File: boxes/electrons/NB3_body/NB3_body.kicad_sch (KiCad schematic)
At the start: 32 parts, among them J1 Conn_02x05_Counter_Clockwise, J10 Conn_02x03_Top_Bottom, J11 Conn_02x03_Top_Bottom, J12 Conn_02x03_Top_Bottom, J13 JST ZH 6-way Socket, J14 JST ZH 6-way Socket, J2 Conn_02x05_Counter_Clockwise, J3 Conn_02x05_Counter_Clockwise, J4 Conn_02x05_Counter_Clockwise, J5 Conn_02x05_Counter_Clockwise, J6 Conn_02x05_Counter_Clockwise, J7 Conn_02x05_Counter_Clockwise, J8 Conn_02x05_Counter_Clockwise, J9 JST SH 4-way Socket

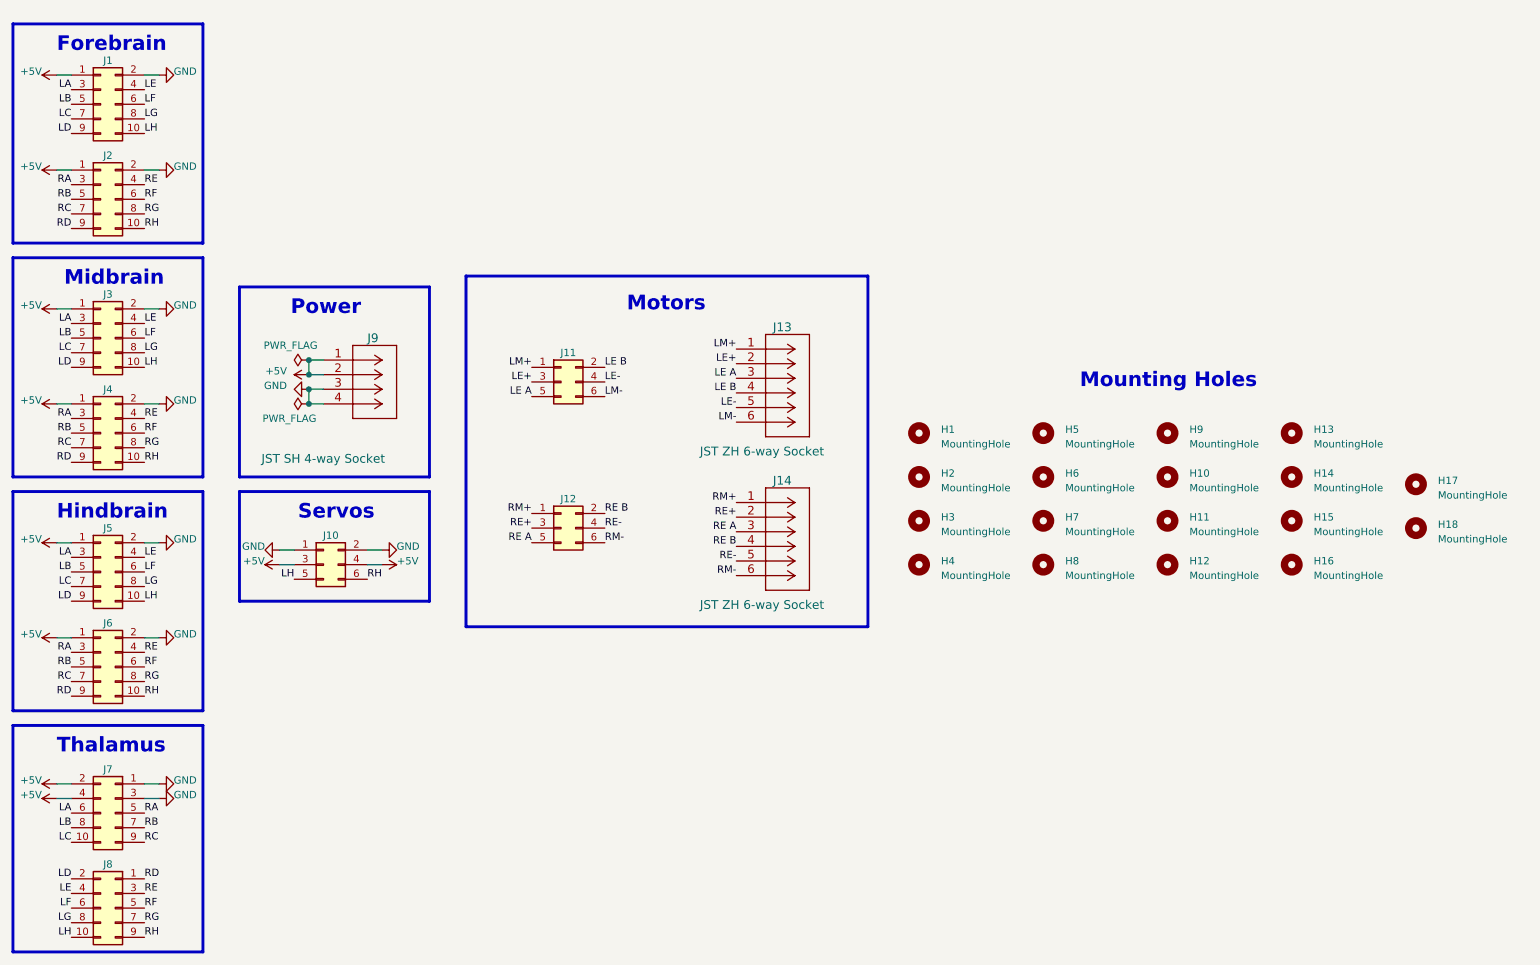
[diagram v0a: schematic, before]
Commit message: Work on NB£_body PCB
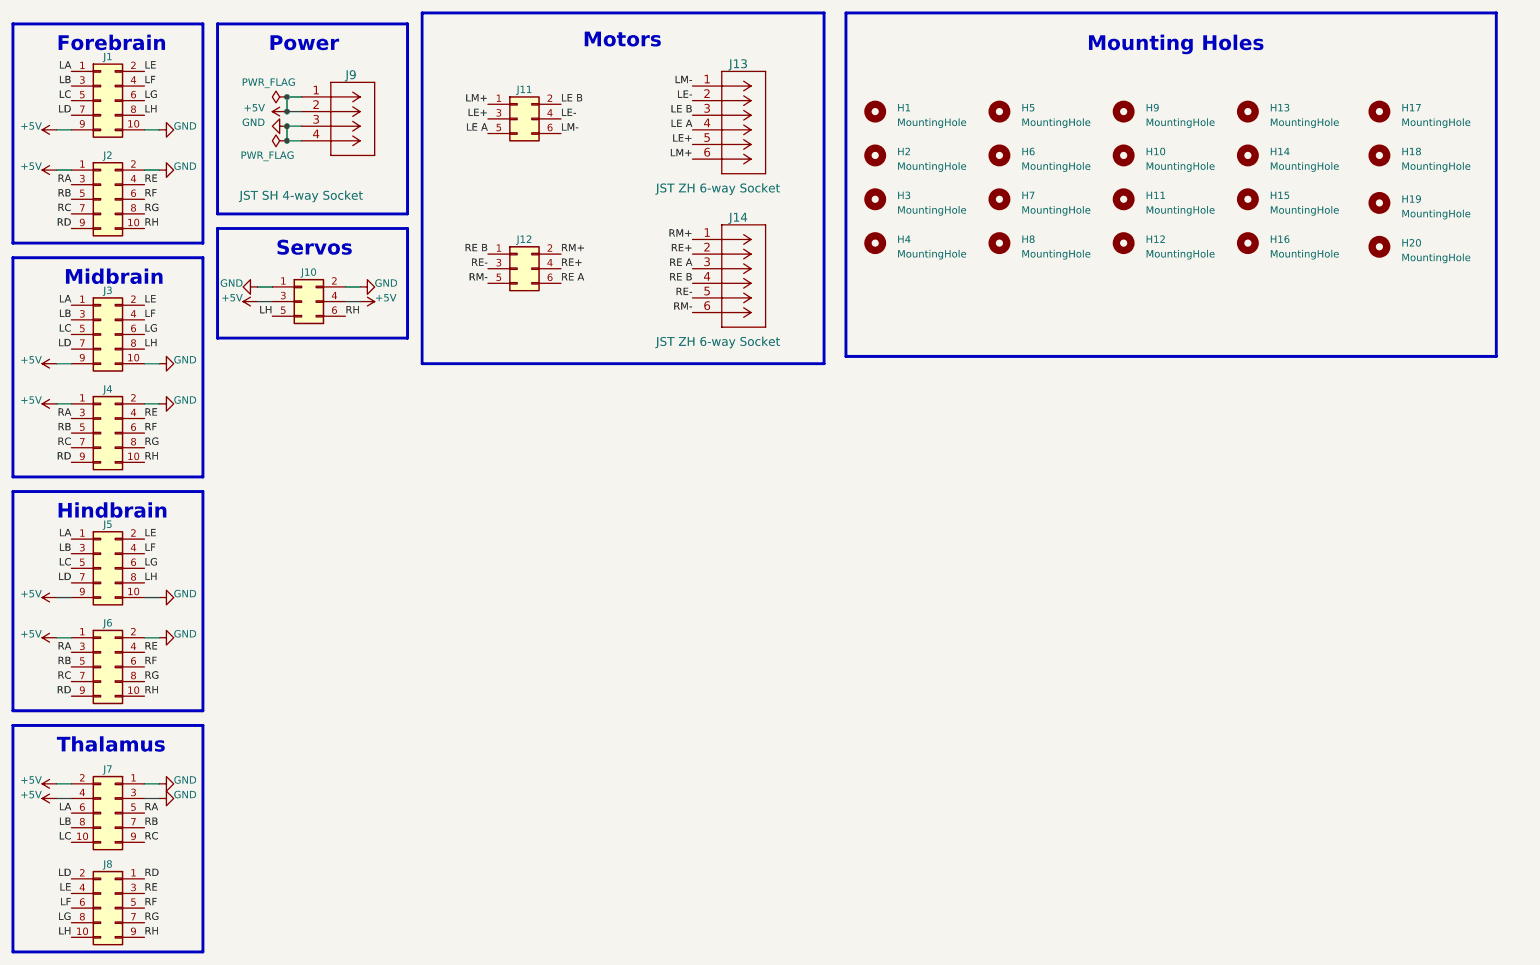
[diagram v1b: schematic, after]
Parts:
- added H19, H20: MountingHole, MountingHole:MountingHole_2.7mm_M2.5_ISO7380_Pad, symbol Mechanical:MountingHole
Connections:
- net +5V: now also J1.9 (Pin_9), J3.9 (Pin_9), J5.9 (Pin_9); no longer J1.1 (Pin_1), J3.1 (Pin_1), J5.1 (Pin_1)
- net GND: now also J1.10 (Pin_10), J3.10 (Pin_10), J5.10 (Pin_10); no longer J1.2 (Pin_2), J3.2 (Pin_2), J5.2 (Pin_2)
- net LA: now also J1.1 (Pin_1), J3.1 (Pin_1), J5.1 (Pin_1); no longer J1.3 (Pin_3), J3.3 (Pin_3), J5.3 (Pin_3)
- net LB: now also J1.3 (Pin_3), J3.3 (Pin_3), J5.3 (Pin_3); no longer J1.5 (Pin_5), J3.5 (Pin_5), J5.5 (Pin_5)
- net LC: now also J1.5 (Pin_5), J3.5 (Pin_5), J5.5 (Pin_5); no longer J1.7 (Pin_7), J3.7 (Pin_7), J5.7 (Pin_7)
- net LD: now also J1.7 (Pin_7), J3.7 (Pin_7), J5.7 (Pin_7); no longer J1.9 (Pin_9), J3.9 (Pin_9), J5.9 (Pin_9)
- net LE: now also J1.2 (Pin_2), J3.2 (Pin_2), J5.2 (Pin_2); no longer J1.4 (Pin_4), J3.4 (Pin_4), J5.4 (Pin_4)
- net LE A: now also J13.4; no longer J13.3
- net LE B: now also J13.3; no longer J13.4
- net LE+: now also J13.5; no longer J13.2
- net LE-: now also J13.2; no longer J13.5
- net LF: now also J1.4 (Pin_4), J3.4 (Pin_4), J5.4 (Pin_4); no longer J1.6 (Pin_6), J3.6 (Pin_6), J5.6 (Pin_6)
- net LG: now also J1.6 (Pin_6), J3.6 (Pin_6), J5.6 (Pin_6); no longer J1.8 (Pin_8), J3.8 (Pin_8), J5.8 (Pin_8)
- net LH: now also J1.8 (Pin_8), J3.8 (Pin_8), J5.8 (Pin_8); no longer J1.10 (Pin_10), J3.10 (Pin_10), J5.10 (Pin_10)
- net LM+: now also J13.6; no longer J13.1
- net LM-: now also J13.1; no longer J13.6
- net RE A: now also J12.6 (Pin_6); no longer J12.5 (Pin_5)
- net RE B: now also J12.1 (Pin_1); no longer J12.2 (Pin_2)
- net RE+: now also J12.4 (Pin_4); no longer J12.3 (Pin_3)
- net RE-: now also J12.3 (Pin_3); no longer J12.4 (Pin_4)
- net RM+: now also J12.2 (Pin_2); no longer J12.1 (Pin_1)
- net RM-: now also J12.5 (Pin_5); no longer J12.6 (Pin_6)
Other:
- moved on the sheet: H1, H10, H11, H12, H13, H14, H15, H16, H17, H18, H2, H3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
